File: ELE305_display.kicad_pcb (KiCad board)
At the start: 2 copper layers, 120.6 x 110.5 mm, 20 parts, among them J2 687124182122

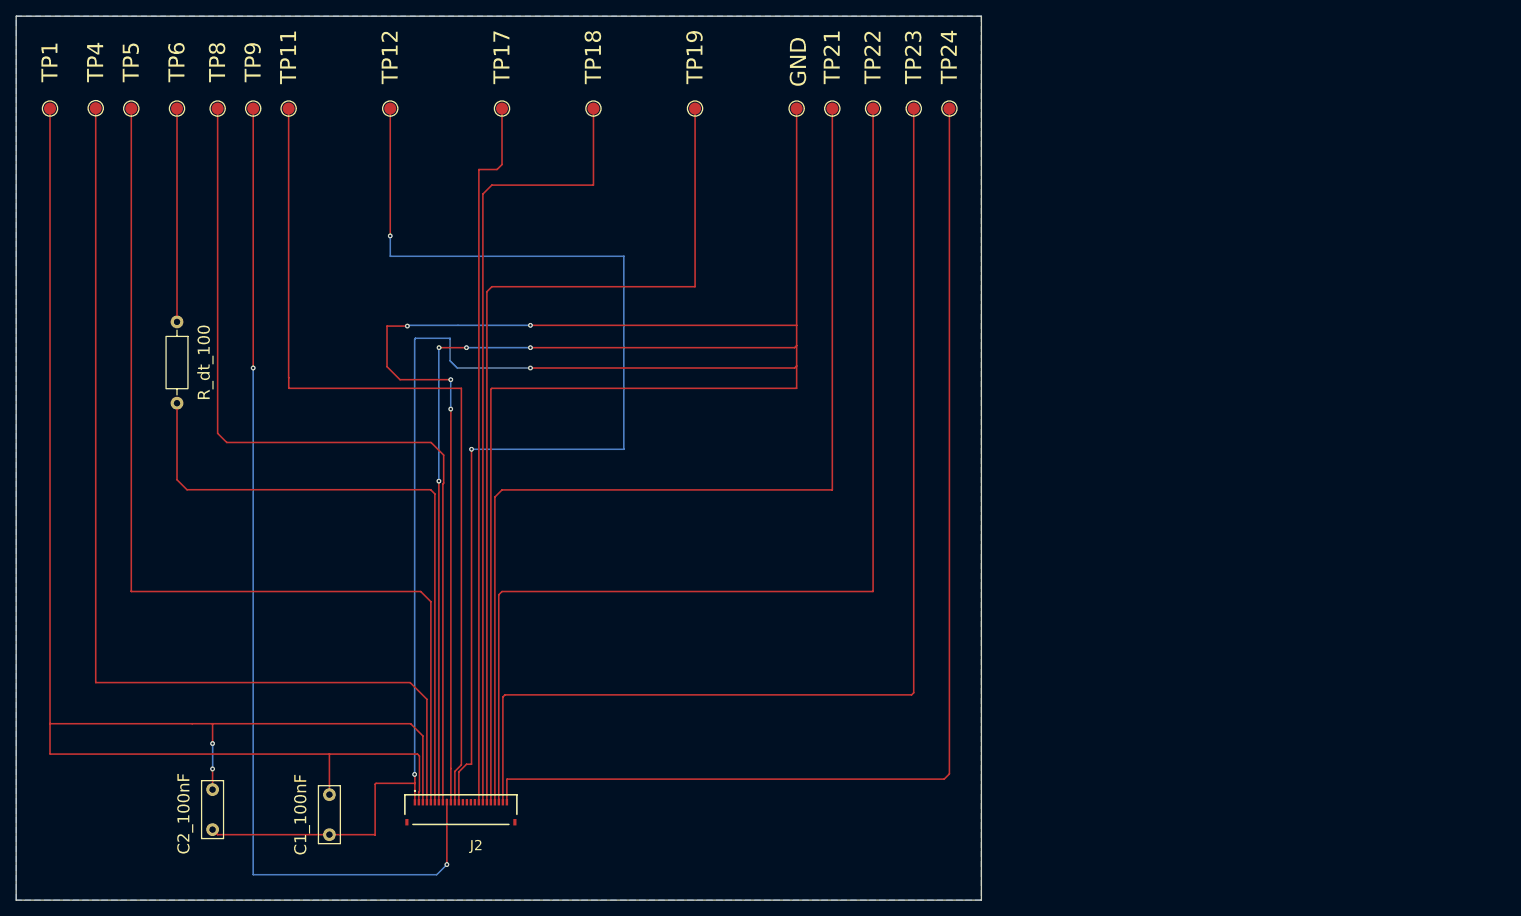
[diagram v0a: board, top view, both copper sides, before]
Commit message: Updated PCB
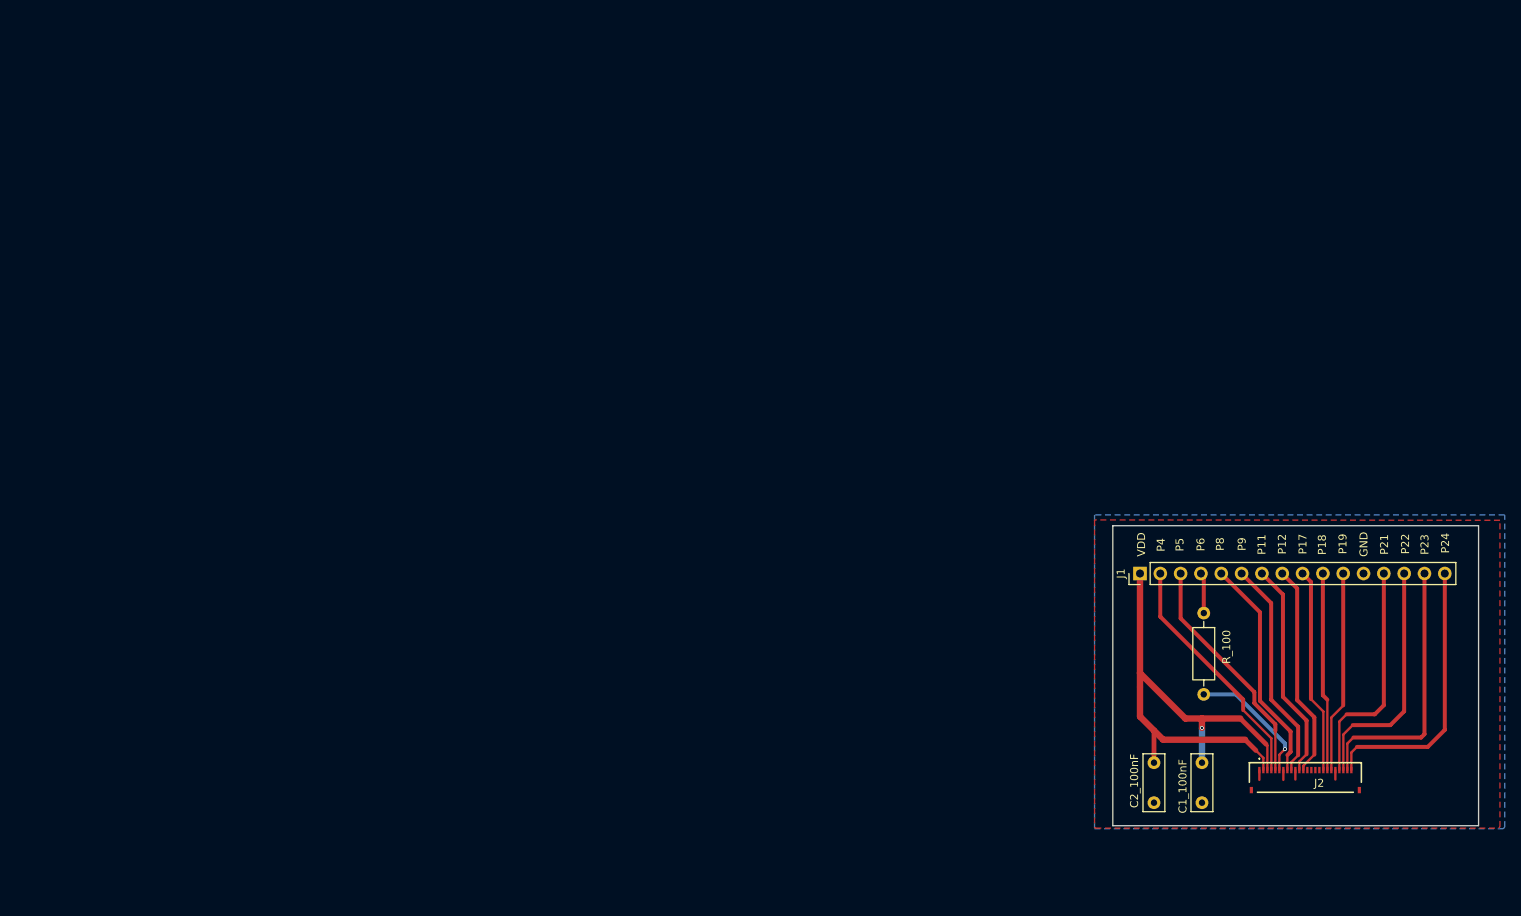
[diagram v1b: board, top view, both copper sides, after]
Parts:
- removed GND: GND, TestPoint:TestPoint_Pad_D1.5mm
- removed TP1: VDD, TestPoint:TestPoint_Pad_D1.5mm
- removed TP11: P11, TestPoint:TestPoint_Pad_D1.5mm
- removed TP12: P12, TestPoint:TestPoint_Pad_D1.5mm
- removed TP17: P17, TestPoint:TestPoint_Pad_D1.5mm
- removed TP18: P18, TestPoint:TestPoint_Pad_D1.5mm
- removed TP19: P19, TestPoint:TestPoint_Pad_D1.5mm
- removed TP21: P21, TestPoint:TestPoint_Pad_D1.5mm
- removed TP22: P22, TestPoint:TestPoint_Pad_D1.5mm
- removed TP23: P23, TestPoint:TestPoint_Pad_D1.5mm
- removed TP24: P24, TestPoint:TestPoint_Pad_D1.5mm
- removed TP4: P4, TestPoint:TestPoint_Pad_D1.5mm
- removed TP5: P5, TestPoint:TestPoint_Pad_D1.5mm
- removed TP6: SDIO, TestPoint:TestPoint_Pad_D1.5mm
- removed TP8: P8, TestPoint:TestPoint_Pad_D1.5mm
- removed TP9: P9, TestPoint:TestPoint_Pad_D1.5mm
- added J1: Conn_01x16_Pin, Connector_PinHeader_2.54mm:PinHeader_1x16_P2.54mm_Vertical, F.Cu at (155.1, 89.3)
- moved R_100 133.4 mm to (163.1, 94.3)
- moved C2_100nF 117.7 mm to (156.8, 118.0)
- moved C1 109.1 mm to (162.8, 118.0)
- moved J2 105.6 mm to (175.8, 114.8)
- renumbered C1_100nF to C1, R_dt_100 to R_100
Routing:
- net GND: track 483.7 -> 4.80 mm, vias 10 -> 0
- net Net-(J1-Pin_1): track 200.9 -> 69.3 mm, vias 2 -> 1
- net Net-(J1-Pin_8): track 135.6 -> 26.8 mm, vias 2 -> 0
- net Net-(J1-Pin_16): track 141.6 -> 34.6 mm
- net Net-(J1-Pin_15): track 137.4 -> 33.5 mm
- net Net-(J1-Pin_14): track 132.9 -> 30.5 mm
- net Net-(J1-Pin_6): track 128.7 -> 27.9 mm, vias 2 -> 0
- net Net-(J1-Pin_13): track 128.0 -> 28.9 mm
- net Net-(J1-Pin_2): track 126.5 -> 30.3 mm
- net Net-(J1-Pin_3): track 123.1 -> 29.5 mm
- net Net-(J1-Pin_11): track 112.0 -> 25.2 mm
- net Net-(J1-Pin_5): track 113.0 -> 28.3 mm
- net Net-(J1-Pin_7): track 108.2 -> 27.3 mm
- net Net-(J1-Pin_10): track 99.5 -> 24.8 mm
- net Net-(J2-Pad6): track 80.7 -> 16.3 mm, vias 0 -> 1
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- added copper zone on F.Cu, net GND
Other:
- board size 120.6 x 110.5 mm -> 45.7 x 37.5 mm
- board text added: "C1_100nF"
- board text added: "GND"
- board text added: "P11"
- board text added: "P12"
- board text added: "P17"
- board text added: "P18"
- board text added: "P19"
- board text added: "P21"
- board text added: "P22"
- board text added: "P23"
- board text added: "P24"
- board text added: "P4"
- board text added: "P5"
- board text added: "P6"
- board text added: "P8"
- board text added: "P9"
- board text added: "VDD"
